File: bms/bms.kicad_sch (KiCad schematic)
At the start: 27 parts, among them J1 Conn_01x16_Pin, J10 Conn_01x02_Pin, J11 Conn_01x02_Pin, J12 Conn_01x02_Pin, J13 Conn_01x02_Pin, J14 Conn_01x08_Pin, J15 Conn_01x08_Pin, J16 Conn_01x02_Pin, J17 Conn_01x08_Pin, J18 Conn_01x08_Pin, J19 Conn_01x08_Pin, J2 Conn_01x16_Pin, J20 Conn_01x08_Pin, J21 Conn_01x08_Pin, J22 Conn_01x08_Socket, J23 Conn_01x10_Socket, J24 Conn_01x08_Pin, J25 Conn_01x02_Pin, J26 Conn_01x06_Socket, J27 Conn_01x06_Socket, J3 Conn_01x02_Pin, J4 Conn_01x02_Pin, J5 Conn_01x02_Pin, J6 Conn_01x16_Pin, J7 Conn_01x20_Pin, J8 Conn_01x20_Pin, J9 Conn_01x02_Pin

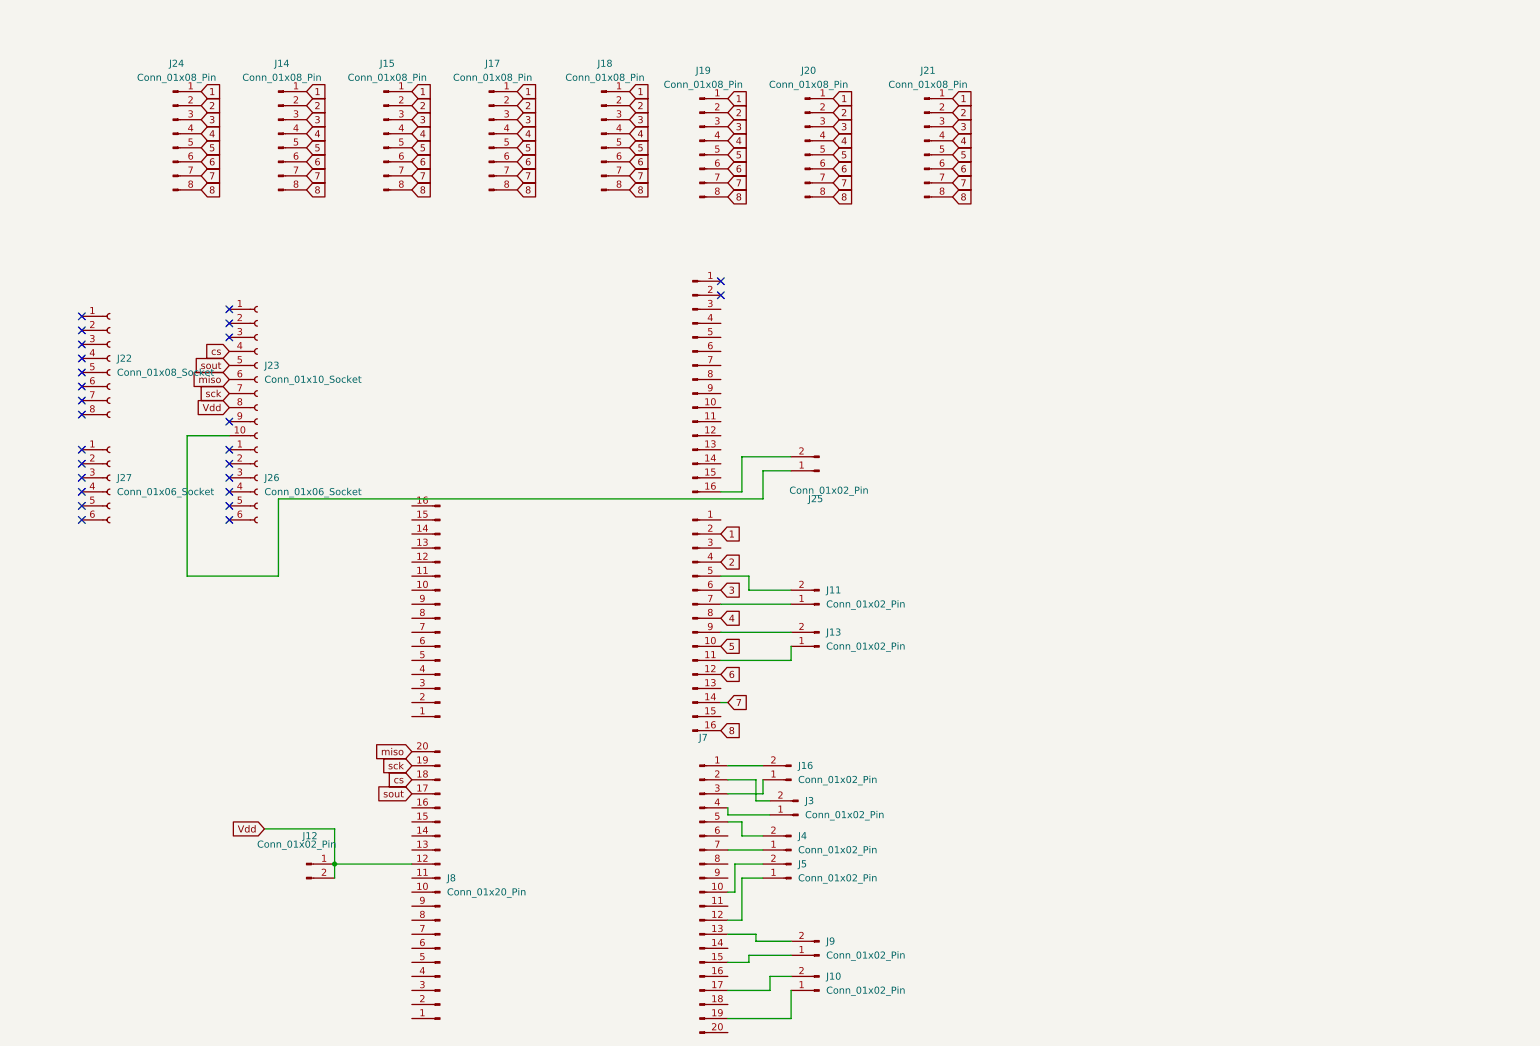
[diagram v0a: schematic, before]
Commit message: prajeala_maxima_3
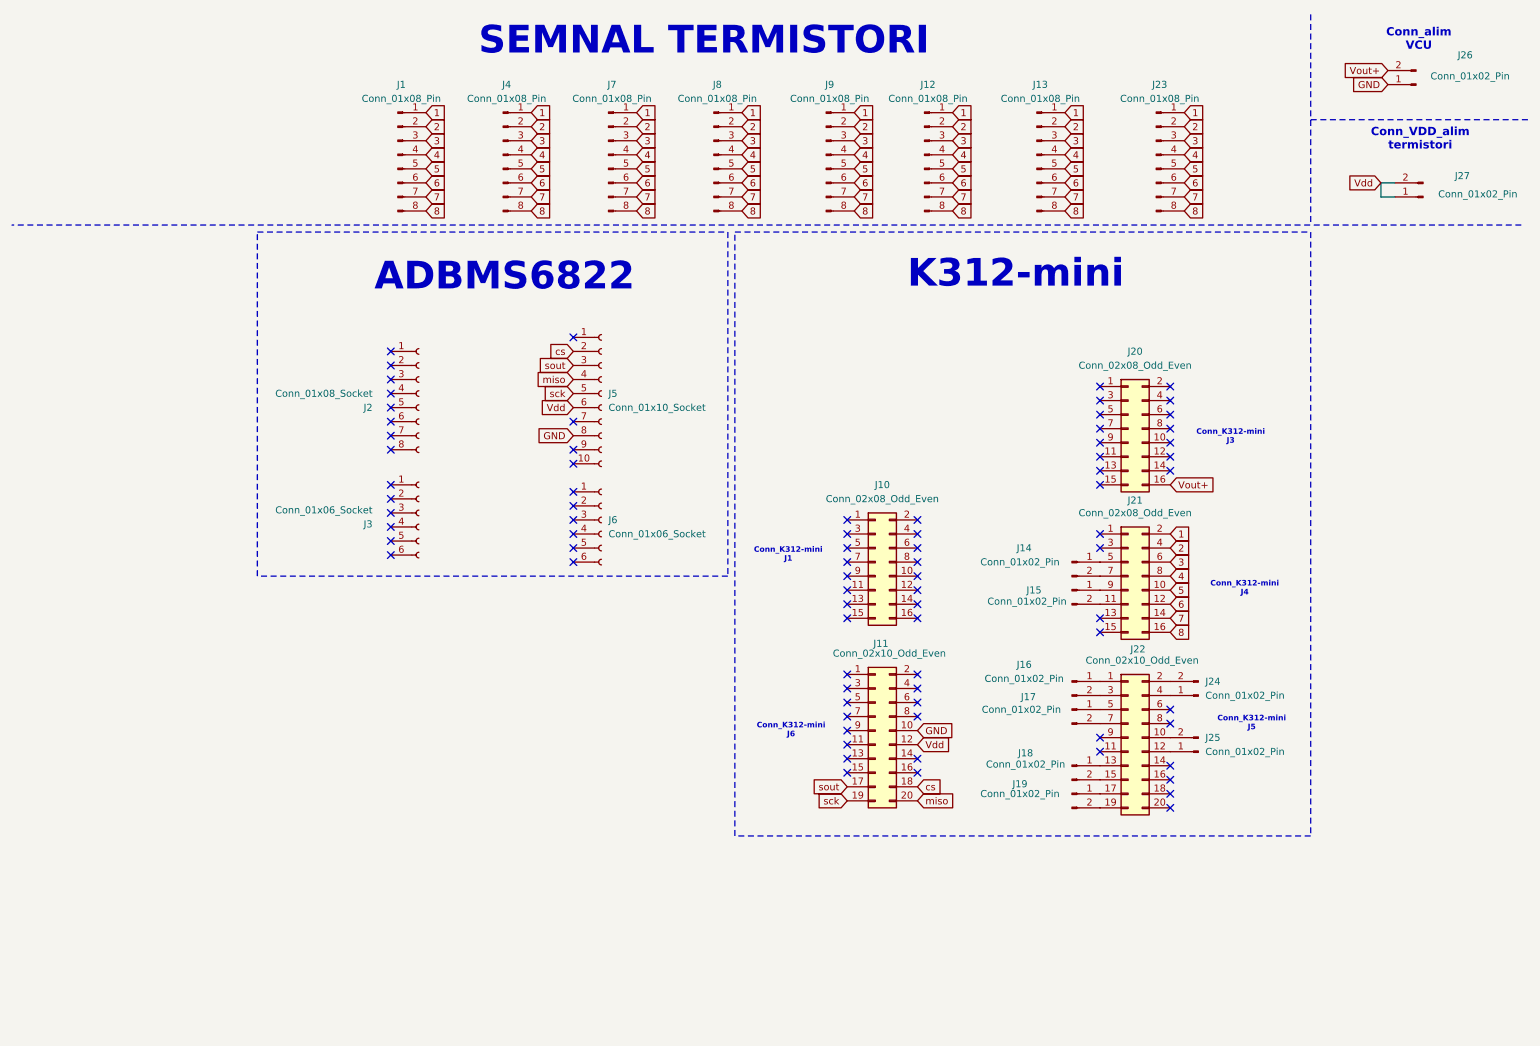
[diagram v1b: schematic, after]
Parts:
- removed J1, J2, J6: Conn_01x16_Pin, Connector_PinHeader_2.54mm:PinHeader_2x08_P2.54mm_Vertical, symbol Connector:Conn_01x16_Pin
- removed J7, J8: Conn_01x20_Pin, Connector_PinHeader_2.54mm:PinHeader_2x10_P2.54mm_Vertical, symbol Connector:Conn_01x20_Pin
- added J10, J20, J21: Conn_02x08_Odd_Even, Connector_PinHeader_2.54mm:PinHeader_2x08_P2.54mm_Vertical, symbol Connector_Generic:Conn_02x08_Odd_Even
- added J11, J22: Conn_02x10_Odd_Even, Connector_PinHeader_2.54mm:PinHeader_2x10_P2.54mm_Vertical, symbol Connector_Generic:Conn_02x10_Odd_Even
- renumbered J24 to J1, J19 to J12, J20 to J13, J11 to J14, J13 to J15, J4 to J17, J9 to J18, J10 to J19, J22 to J2, J21 to J23, J3 to J24, J5 to J25, J25 to J26, J12 to J27, J27 to J3, J14 to J4, J23 to J5, J26 to J6, J15 to J7, J17 to J8, J18 to J9
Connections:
- net 1: now also J21.2 (Pin_2)
- net 2: now also J21.4 (Pin_4)
- net 3: now also J21.6 (Pin_6)
- net 4: now also J21.8 (Pin_8)
- net 5: now also J21.10 (Pin_10)
- net 6: now also J21.12 (Pin_12)
- net 7: now also J21.14 (Pin_14)
- net 8: now also J21.16 (Pin_16)
- net Vdd: now also J5.6 (Pin_6), J11.12 (Pin_12); no longer J5.8 (Pin_8)
- net cs: now also J5.2 (Pin_2), J11.18 (Pin_18); no longer J5.4 (Pin_4)
- net miso: now also J5.4 (Pin_4), J11.20 (Pin_20); no longer J5.6 (Pin_6)
- net sck: now also J5.5 (Pin_5), J11.19 (Pin_19); no longer J5.7 (Pin_7)
- net sout: now also J5.3 (Pin_3), J11.17 (Pin_17); no longer J5.5 (Pin_5)
- net at J25.1 (Pin_1): now also J22.12 (Pin_12)
- net at J25.2 (Pin_2): now also J22.10 (Pin_10)
- net at J14.1 (Pin_1): now also J21.5 (Pin_5)
- net at J14.2 (Pin_2): now also J21.7 (Pin_7)
- net at J19.1 (Pin_1): now also J22.17 (Pin_17)
- net at J19.2 (Pin_2): now also J22.19 (Pin_19)
- net at J18.1 (Pin_1): now also J22.13 (Pin_13)
- net at J18.2 (Pin_2): now also J22.15 (Pin_15)
- net at J24.1 (Pin_1): now also J22.4 (Pin_4)
- net at J24.2 (Pin_2): now also J22.2 (Pin_2)
- net at J16.2 (Pin_2): now also J22.3 (Pin_3)
- net at J16.1 (Pin_1): now also J22.1 (Pin_1)
- net at J17.2 (Pin_2): now also J22.7 (Pin_7)
- net at J17.1 (Pin_1): now also J22.5 (Pin_5)
- net at J15.1 (Pin_1): now also J21.9 (Pin_9)
- net at J15.2 (Pin_2): now also J21.11 (Pin_11)
- net Vout+: now reaches J26.2 (Pin_2)
- net Vout+: now also J20.16 (Pin_16)
- net at J5.10 (Pin_10): no longer J26.1 (Pin_1)
- new net GND: J11.10 (Pin_10), J26.1 (Pin_1), J5.8 (Pin_8)
- no-connect marks 26 -> 81
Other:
- note added: "ADBMS6822"
- note added: "Conn_K312-mini J1"
- note added: "Conn_K312-mini J3"
- note added: "Conn_K312-mini J4"
- note added: "Conn_K312-mini J5"
- note added: "Conn_K312-mini J6"
- note added: "Conn_VDD_alim termistori"
- note added: "Conn_alim VCU"
- note added: "K312-mini"
- note added: "SEMNAL TERMISTORI"
- moved on the sheet: J1, J12, J13, J14, J15, J16, J17, J18, J19, J2, J23, J24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
